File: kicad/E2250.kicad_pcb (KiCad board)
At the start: 2 copper layers, 22 x 46 mm, 2 parts

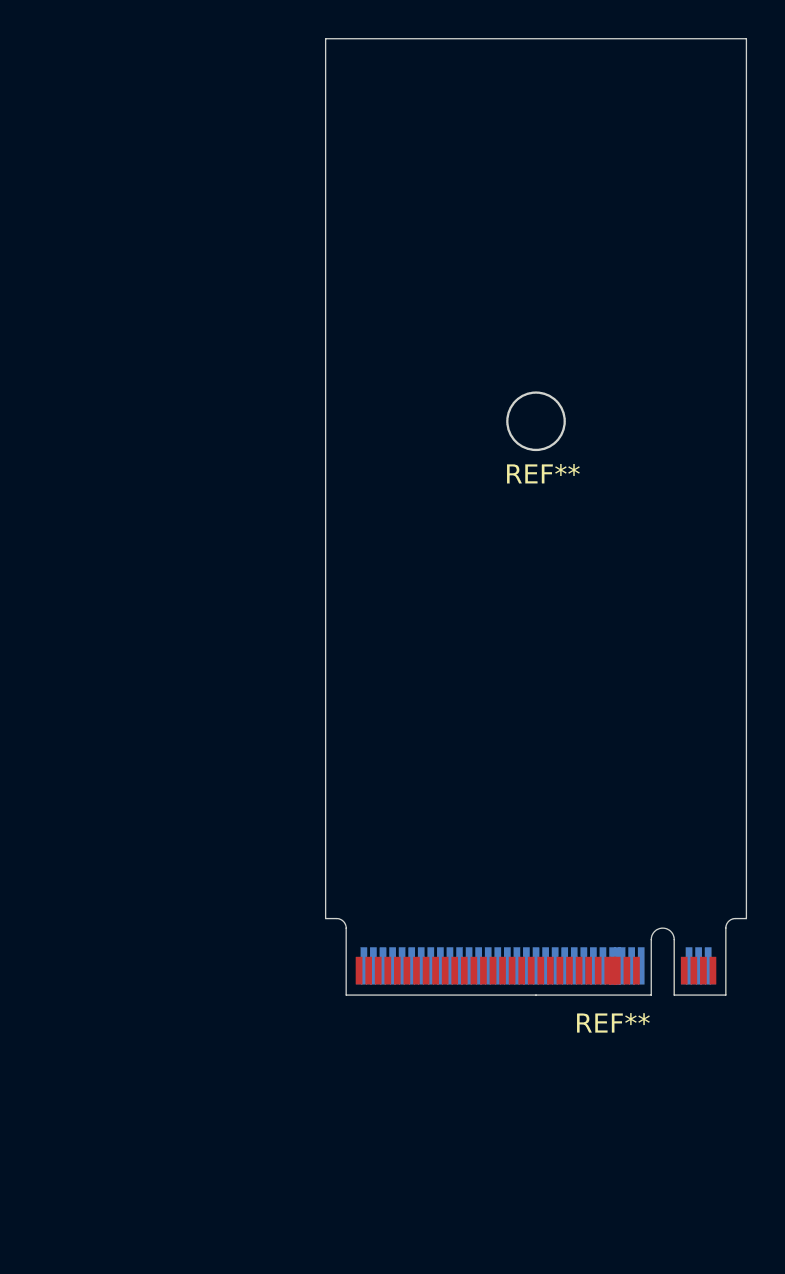
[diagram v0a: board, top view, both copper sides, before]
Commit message: update
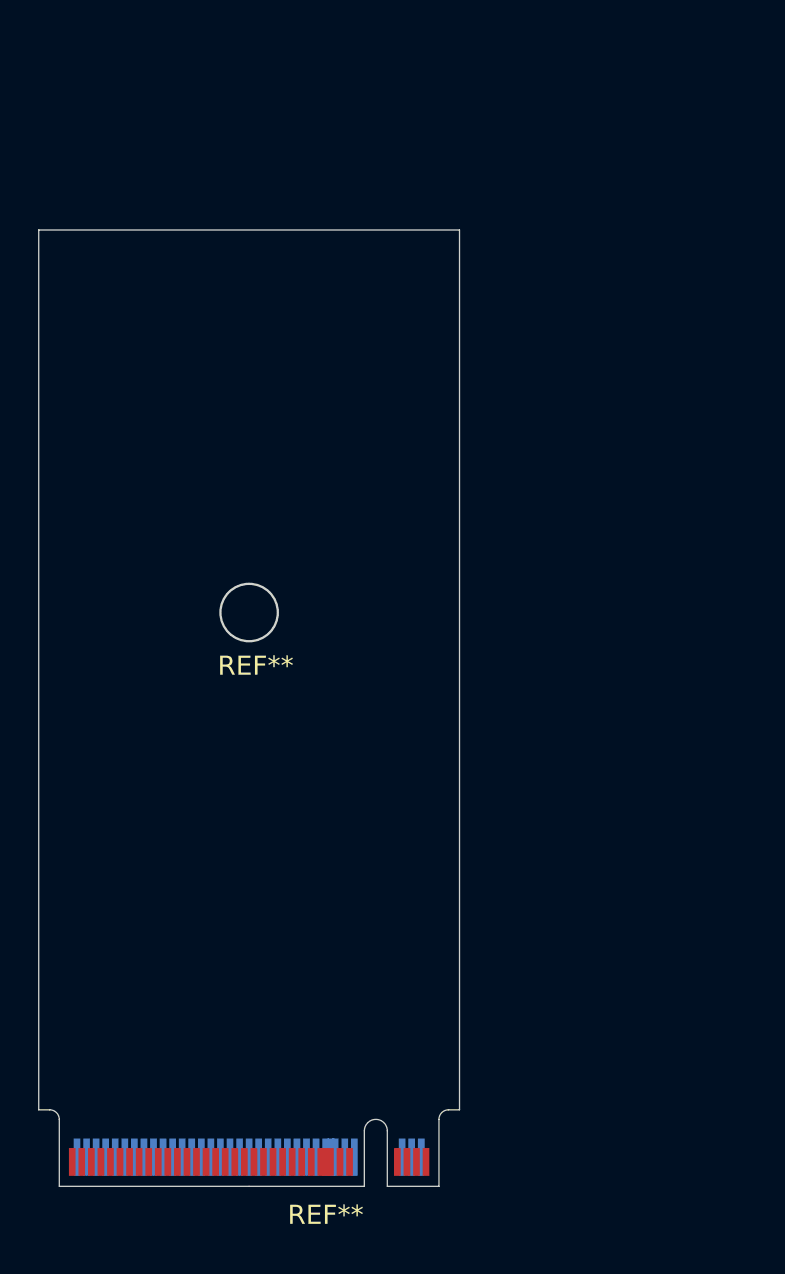
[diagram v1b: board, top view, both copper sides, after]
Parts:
- moved NGFF2250 18.0 mm to (100.0, 100.0)
- moved REF** 18.0 mm to (100.0, 100.0)
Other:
- rule pad_to_mask_clearance: 0.051 -> 0.05
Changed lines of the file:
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@@
 (kicad_pcb (version 20211014) (generator pcbnew)
   (general
-    (thickness 1.6)
+    (thickness 0.8)
   )
   (paper "A4")
@@
   )
   (setup
-    (pad_to_mask_clearance 0.051)
+    (pad_to_mask_clearance 0.05)
     (solder_mask_min_width 0.25)
+    (aux_axis_origin 100 100)
+    (grid_origin 100 100)
     (pcbplotparams
       (layerselection 0x00010fc_ffffffff)
@@
   (net 0 "")
   (footprint "ngff:NGFF_A" (layer "F.Cu")
-    (at 115 90)
+    (at 100 100)
     (attr through_hole)
     (fp_text reference "REF**" (at 4 1.5) (layer "F.SilkS")
@@
   )
   (footprint "ngff:NGFF_2250" (layer "F.Cu")
-    (at 115 90)
+    (at 100 100)
     (attr through_hole)
     (fp_text reference "NGFF2250" (at -0.05 -25.92) (layer "F.Fab")
